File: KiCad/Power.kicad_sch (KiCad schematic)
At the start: 17 parts, among them Q1 PMOS, Q2 NMOS, Q3 NMOS, Q4 PMOS, SW3 SW_SPDT, U3 ${SIM.PARAMS}, U4 IFX27001TFV

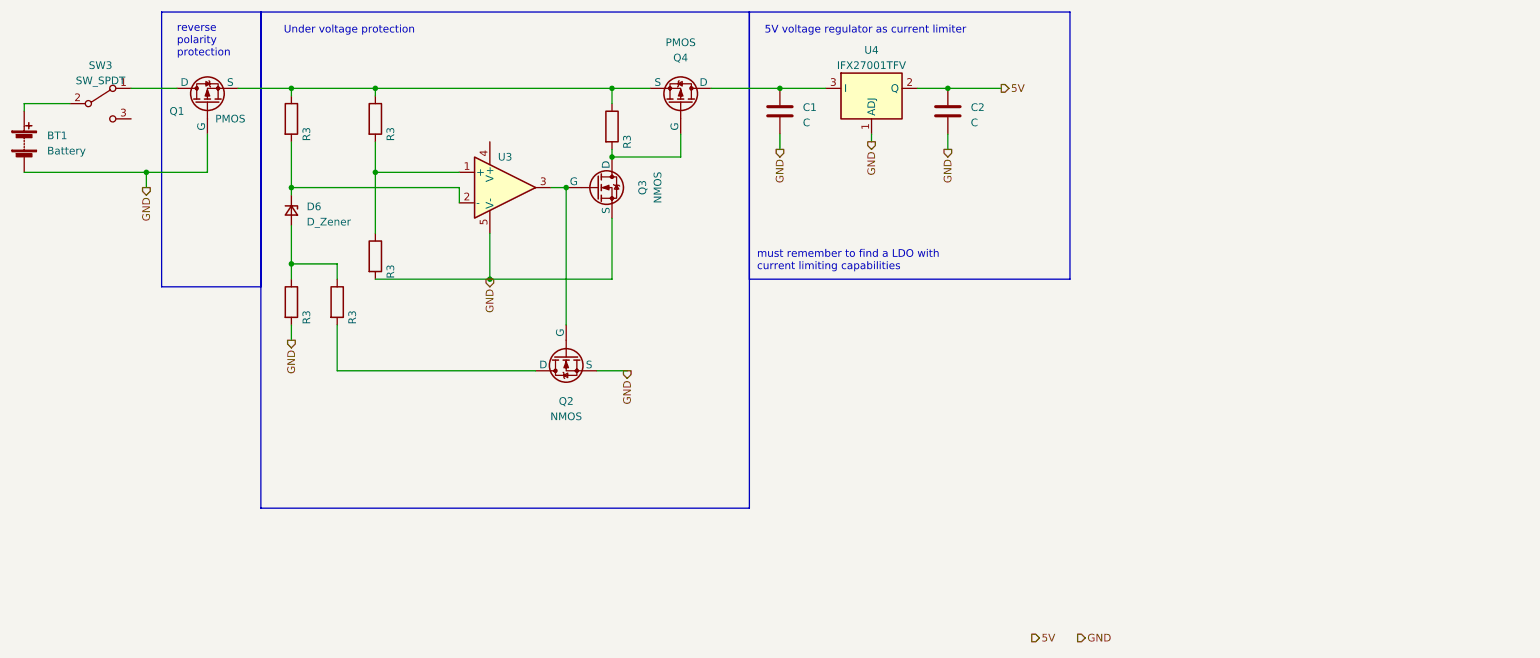
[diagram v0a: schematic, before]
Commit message: ki cad changes
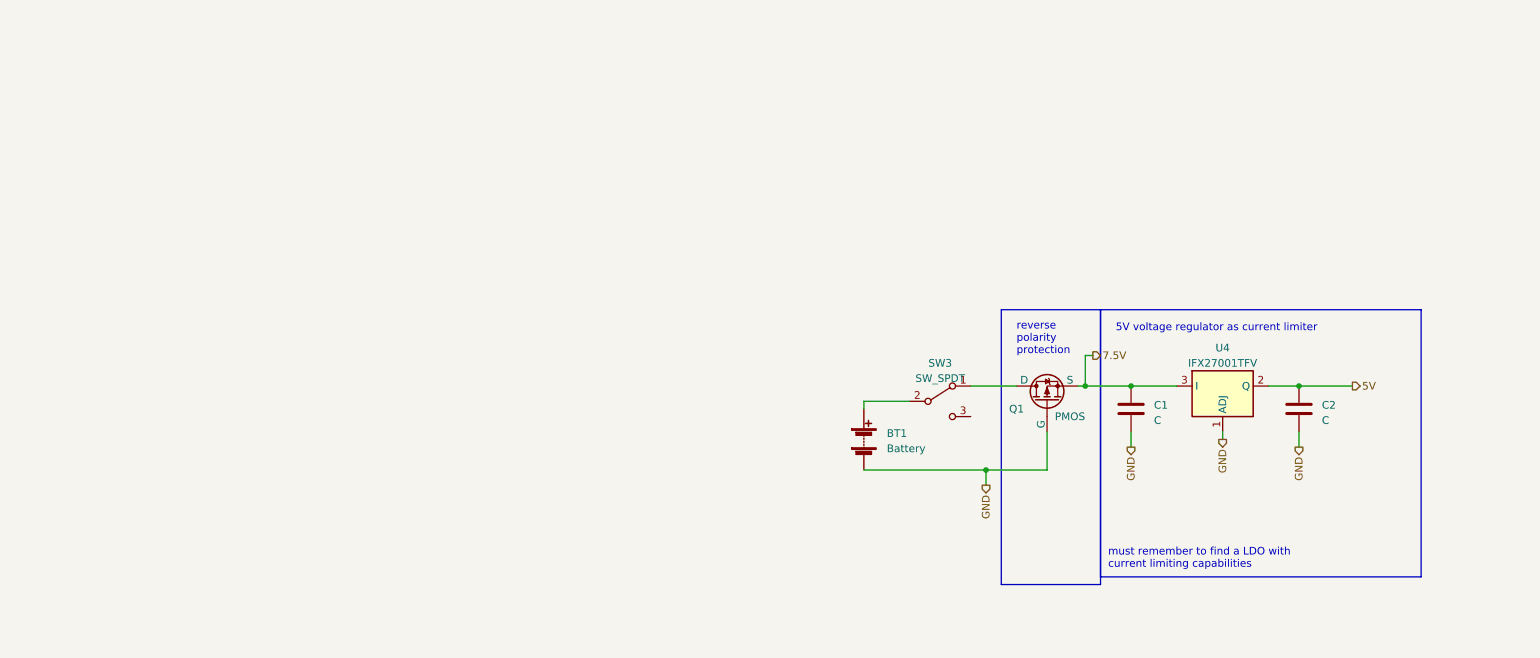
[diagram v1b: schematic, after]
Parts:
- removed D6: D_Zener, symbol Device:D_Zener_Small
- removed Q2, Q3: NMOS, symbol Simulation_SPICE:NMOS
- removed Q4: PMOS, symbol Simulation_SPICE:PMOS
- removed R3 (x6): ~, symbol Device:R
- removed U3: ${SIM.PARAMS}, symbol Simulation_SPICE:OPAMP
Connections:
- net 7.5V: now reaches Q1.3 (S)
- net 7.5V: now also C1.1, U4.3 (I)
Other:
- note removed: "Under voltage protection"
- moved on the sheet: BT1, C1, C2, Q1, SW3, U4

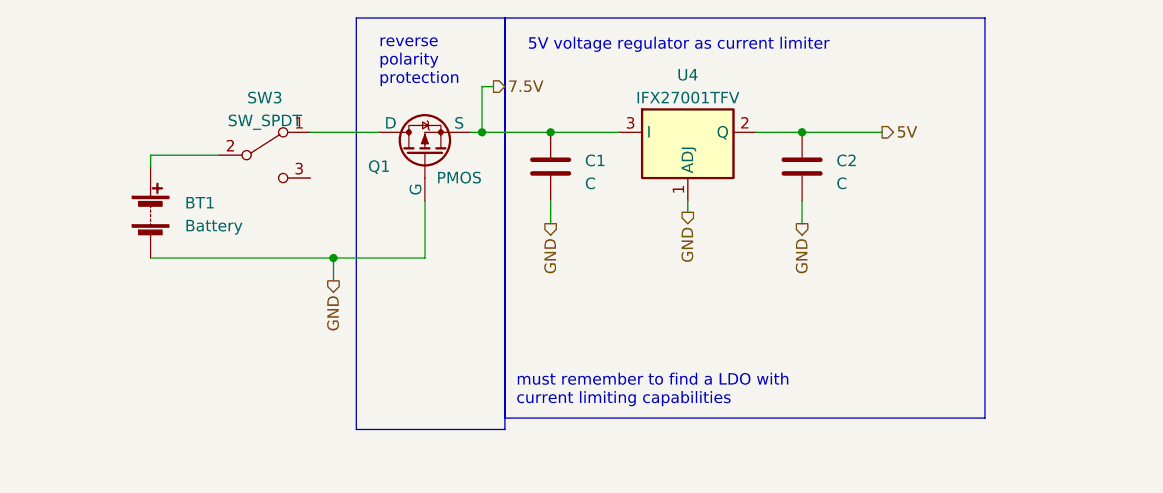
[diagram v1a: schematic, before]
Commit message: kicad
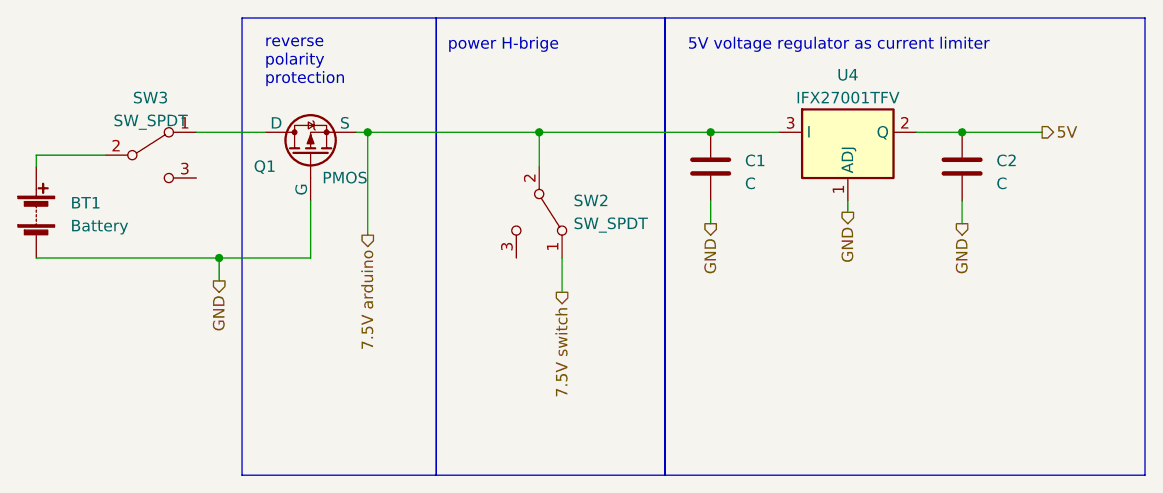
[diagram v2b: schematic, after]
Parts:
- added SW2: SW_SPDT, symbol Switch:SW_SPDT
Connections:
- net 7.5V renamed 7.5V arduino
- net 7.5V arduino: now also SW2.2 (B)
- new net 7.5V switch: SW2.1 (A)
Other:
- note added: "power H-brige"
- note removed: "must remember to find a LDO with current limiting capabilities"
- moved on the sheet: BT1, C1, C2, Q1, SW3, U4
